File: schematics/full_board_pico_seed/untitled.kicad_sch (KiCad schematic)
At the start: 10 parts, among them J4 Conn_01x03_Female, U4 LM4881M/NOPB

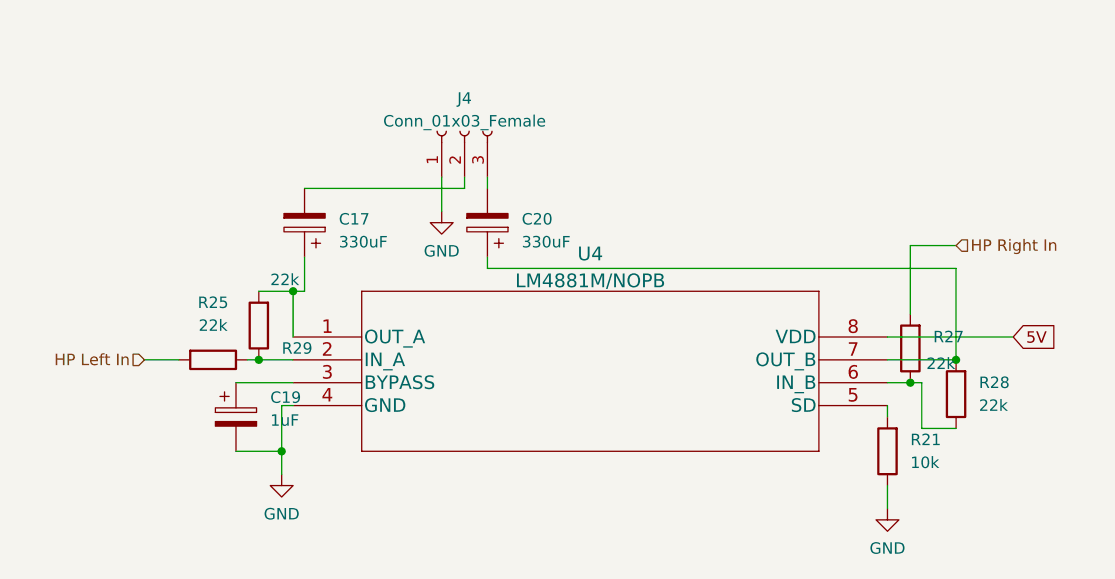
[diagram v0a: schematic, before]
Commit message: schematic change
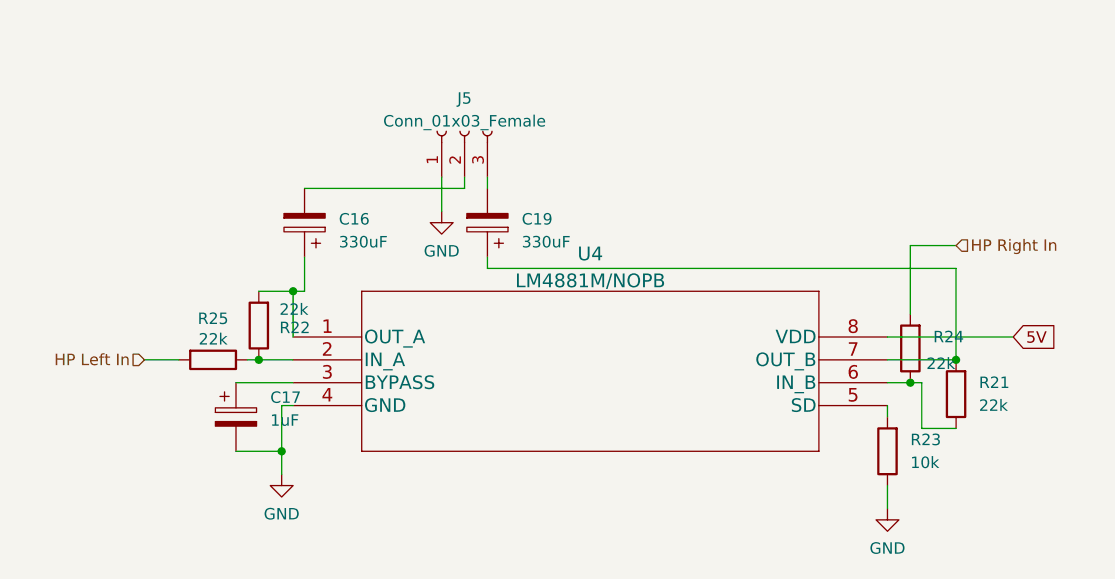
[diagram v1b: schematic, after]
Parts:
- renumbered C17 to C16, C19 to C17, C20 to C19, J4 to J5, R28 to R21, R29 to R22, R21 to R23, R27 to R24
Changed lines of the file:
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@@
 		(on_board yes)
 		(dnp no)
-		(fields_autoplaced yes)
 		(property "Reference" "R25"
-			(at 95.25 53.34 90)
+			(at 95.25 55.118 90)
 			(effects
 				(font
@@
 		)
 		(property "Value" "22k"
-			(at 95.25 55.88 90)
+			(at 95.25 57.404 90)
 			(effects
 				(font
@@
 		(on_board yes)
 		(dnp no)
-		(property "Reference" "R27"
+		(property "Reference" "R24"
 			(at 175.26 57.15 0)
 			(effects
@@
 			(project "full_board_pico_seed"
 				(path "/e63e39d7-6ac0-4ffd-8aa3-1841a4541b55/5b76a2fc-3494-4cf0-b601-f44157bc070a"
-					(reference "R27")
+					(reference "R24")
 					(unit 1)
 				)
@@
 		(on_board yes)
 		(dnp no)
-		(property "Reference" "R29"
-			(at 102.87 58.42 0)
+		(property "Reference" "R22"
+			(at 102.616 56.134 0)
 			(effects
 				(font
@@
 		)
 		(property "Value" "22k"
-			(at 101.6 50.8 0)
+			(at 102.616 54.102 0)
 			(effects
 				(font
@@
 			(project "full_board_pico_seed"
 				(path "/e63e39d7-6ac0-4ffd-8aa3-1841a4541b55/5b76a2fc-3494-4cf0-b601-f44157bc070a"
-					(reference "R29")
+					(reference "R22")
 					(unit 1)
 				)
@@
 		(dnp no)
 		(fields_autoplaced yes)
-		(property "Reference" "R21"
+		(property "Reference" "R23"
 			(at 172.72 68.58 0)
 			(effects
@@
 			(project "full_board_pico_seed"
 				(path "/e63e39d7-6ac0-4ffd-8aa3-1841a4541b55/5b76a2fc-3494-4cf0-b601-f44157bc070a"
-					(reference "R21")
+					(reference "R23")
 					(unit 1)
 				)
@@
 		(dnp no)
 		(fields_autoplaced yes)
-		(property "Reference" "J4"
+		(property "Reference" "J5"
 			(at 123.19 30.641 90)
 			(effects
@@
 			(project "full_board_pico_seed"
 				(path "/e63e39d7-6ac0-4ffd-8aa3-1841a4541b55/5b76a2fc-3494-4cf0-b601-f44157bc070a"
-					(reference "J4")
+					(reference "J5")
 					(unit 1)
 				)
@@
 		(dnp no)
 		(fields_autoplaced yes)
-		(property "Reference" "C17"
+		(property "Reference" "C16"
 			(at 109.22 44.069 0)
 			(effects
@@
 			(project "full_board_pico_seed"
 				(path "/e63e39d7-6ac0-4ffd-8aa3-1841a4541b55/5b76a2fc-3494-4cf0-b601-f44157bc070a"
-					(reference "C17")
+					(reference "C16")
 					(unit 1)
 				)
@@
 		(dnp no)
 		(fields_autoplaced yes)
-		(property "Reference" "C20"
+		(property "Reference" "C19"
 			(at 129.54 44.069 0)
 			(effects
@@
 			(project "full_board_pico_seed"
 				(path "/e63e39d7-6ac0-4ffd-8aa3-1841a4541b55/5b76a2fc-3494-4cf0-b601-f44157bc070a"
-					(reference "C20")
+					(reference "C19")
 					(unit 1)
 				)
@@
 		(dnp no)
 		(fields_autoplaced yes)
-		(property "Reference" "C19"
+		(property "Reference" "C17"
 			(at 101.6 63.881 0)
 			(effects
@@
 			(project "full_board_pico_seed"
 				(path "/e63e39d7-6ac0-4ffd-8aa3-1841a4541b55/5b76a2fc-3494-4cf0-b601-f44157bc070a"
-					(reference "C19")
+					(reference "C17")
 					(unit 1)
 				)
@@
 		(dnp no)
 		(fields_autoplaced yes)
-		(property "Reference" "R28"
+		(property "Reference" "R21"
 			(at 180.34 62.23 0)
 			(effects
@@
 			(project "full_board_pico_seed"
 				(path "/e63e39d7-6ac0-4ffd-8aa3-1841a4541b55/5b76a2fc-3494-4cf0-b601-f44157bc070a"
-					(reference "R28")
-					(unit 1)
-				)
+					(reference "R21")
+					(unit 1)
+				)

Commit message: updated schematic
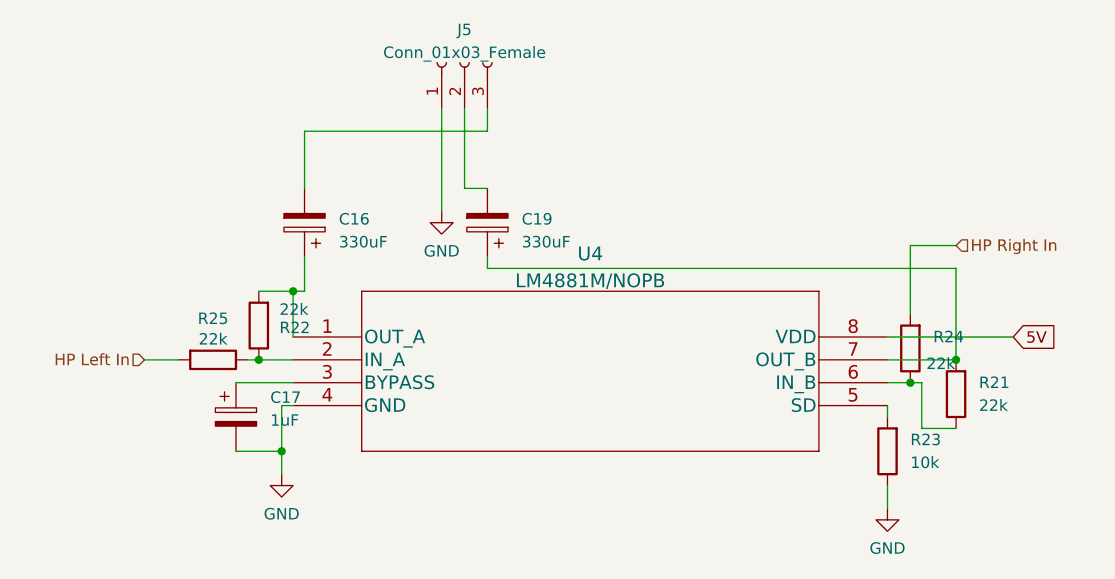
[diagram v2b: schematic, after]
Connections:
- net at J5.2 (Pin_2): now also C19.2; no longer C16.2
- net at J5.3 (Pin_3): now also C16.2; no longer C19.2
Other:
- moved on the sheet: J5
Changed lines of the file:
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@@
+	(wire
+		(pts
+			(xy 123.19 40.64) (xy 123.19 31.75)
+		)
+		(stroke
+			(width 0)
+			(type default)
+		)
+	)
 	(wire
 		(pts
@@
 	(wire
 		(pts
-			(xy 105.41 40.64) (xy 123.19 40.64)
-		)
-		(stroke
-			(width 0)
-			(type default)
-		)
-	)
-	(wire
-		(pts
 			(xy 172.72 46.99) (xy 177.8 46.99)
 		)
@@
 	(wire
 		(pts
-			(xy 125.73 40.64) (xy 125.73 39.37)
+			(xy 125.73 40.64) (xy 123.19 40.64)
 		)
 		(stroke
@@
 	(wire
 		(pts
-			(xy 123.19 40.64) (xy 123.19 39.37)
-		)
-		(stroke
-			(width 0)
-			(type default)
-		)
-	)
-	(wire
-		(pts
 			(xy 177.8 59.69) (xy 177.8 49.53)
 		)
@@
 	(wire
 		(pts
-			(xy 120.65 39.37) (xy 120.65 43.18)
+			(xy 120.65 31.75) (xy 120.65 43.18)
+		)
+		(stroke
+			(width 0)
+			(type default)
+		)
+	)
+	(wire
+		(pts
+			(xy 105.41 34.29) (xy 125.73 34.29)
+		)
+		(stroke
+			(width 0)
+			(type default)
+		)
+	)
+	(wire
+		(pts
+			(xy 105.41 40.64) (xy 105.41 34.29)
+		)
+		(stroke
+			(width 0)
+			(type default)
+		)
+	)
+	(wire
+		(pts
+			(xy 125.73 34.29) (xy 125.73 31.75)
 		)
 		(stroke
@@
 	(symbol
 		(lib_id "Connector:Conn_01x03_Female")
-		(at 123.19 34.29 90)
+		(at 123.19 26.67 90)
 		(unit 1)
 		(exclude_from_sim no)
@@
 		(fields_autoplaced yes)
 		(property "Reference" "J5"
-			(at 123.19 30.641 90)
+			(at 123.19 23.021 90)
 			(effects
 				(font
@@
 		)
 		(property "Value" "Conn_01x03_Female"
-			(at 123.19 33.1779 90)
+			(at 123.19 25.5579 90)
 			(effects
 				(font
@@
 		)
 		(property "Footprint" "Connector_PinHeader_2.54mm:PinHeader_1x03_P2.54mm_Vertical"
-			(at 123.19 34.29 0)
+			(at 123.19 26.67 0)
 			(effects
 				(font
@@
 		)
 		(property "Datasheet" "~"
-			(at 123.19 34.29 0)
+			(at 123.19 26.67 0)
 			(effects
 				(font
@@
 		)
 		(property "Description" ""
-			(at 123.19 34.29 0)
-			(effects
-				(font
+			(at 123.19 26.67 0)
+			(effects
+				(font
